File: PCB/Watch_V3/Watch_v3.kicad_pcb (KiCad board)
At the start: 2 copper layers, 39.1 x 63.2 mm, 102 parts, among them J1 USB_C_Receptacle_USB2.0_16P, J2 Screw_Terminal, J3 Peripheral, J4 OLED, J5 BN220, J6 Peripheral, J7 MAX30102, J8 ICSP, M1 Motor_DC, Q1 AO3401A, Q2 BC817, Q3 BC817, Q4 SI2302, Q5 BC847, SW1 SW_DPST_x2, SW2 SW_SPDT, SW3 SW_DPST_x2, SW4 Mode, SW5 Down, SW6 Select, SW7 Up, U1 AP2112K-3.3, U2 AP2112K-3.3, U3 TP4056, U4 ESP32-WROOM-32D, U5 CP2102N-Axx-xQFN28, U6 MPU-6050

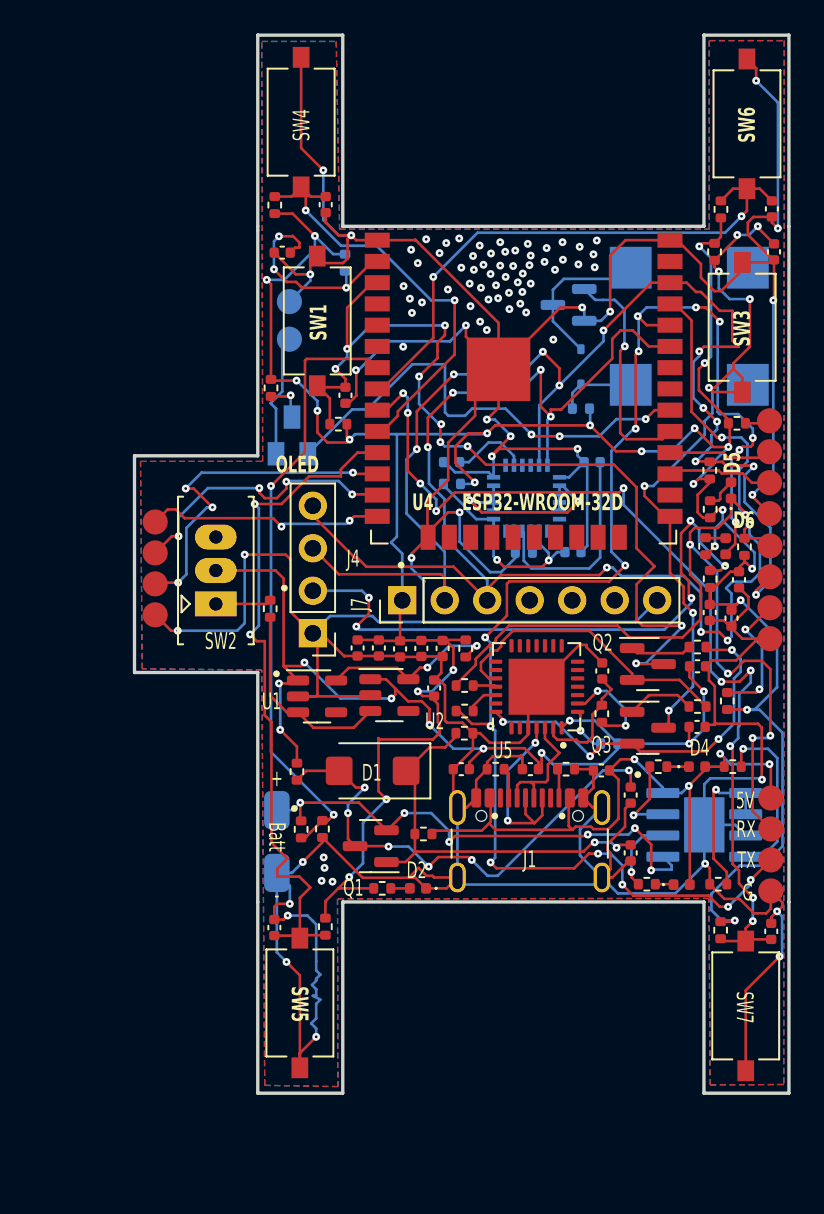
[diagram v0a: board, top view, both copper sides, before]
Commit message: update watch_v3
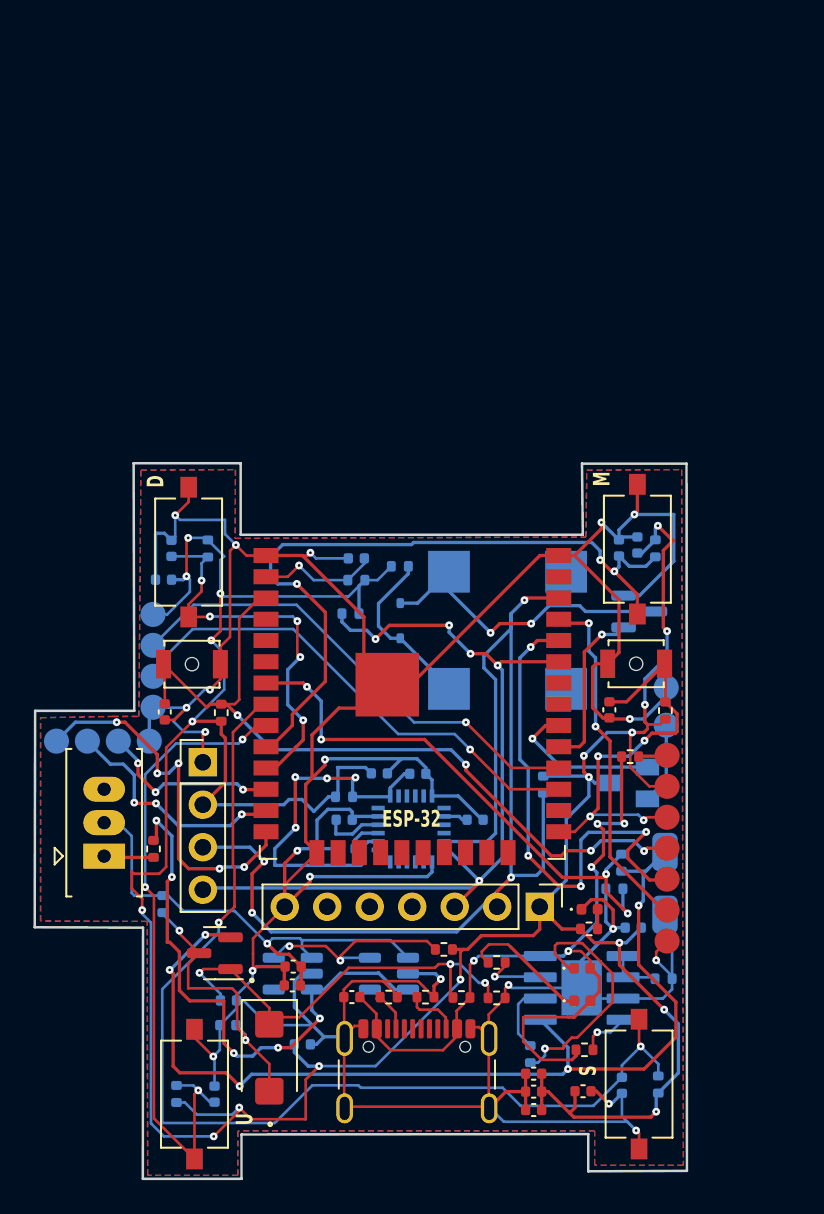
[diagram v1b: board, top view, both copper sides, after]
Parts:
- removed C4, C5, C6: 0.1uF, Capacitor_SMD:C_0402_1005Metric
- removed D5, D6: LED, LED_SMD:LED_0402_1005Metric
- removed G***: LOGO, Battery:xx
- removed G***: LOGO, Battery:robo2
- removed J6: Peripheral, Button_Switch_SMD:solder_pad_4
- removed Q2, Q3: BC817, Package_TO_SOT_SMD:SOT-23
- removed R10, R11: 150E, Resistor_SMD:R_0402_1005Metric
- removed R26, R27, R33, R37, R39: 0, Resistor_SMD:R_0402_1005Metric
- removed R30, R31: 220E, Resistor_SMD:R_0402_1005Metric
- removed R32: 4.7K, Resistor_SMD:R_0402_1005Metric
- removed R8: 1K, Resistor_SMD:R_0402_1005Metric
- removed U5: CP2102N-Axx-xQFN28, Package_DFN_QFN:QFN-28-1EP_5x5mm_P0.5mm_EP3.35x3.35mm
- C10, C11, C12, C17, C18, C2, C25, C26, C27, C28, C3, C9, J3, J5, R14, R15, R16, R17, R21, R22, R23, R24, R34, R5, R7, U1, U2: moved to B.Cu
- J8: value ICSP -> Conn_01x07_Pin; footprint Button_Switch_SMD:solder_pad_4 -> Button_Switch_SMD:solder_7
- R9: value 1K -> 0
- SW1, SW3: footprint Button_Switch_SMD:SW_Tactile_SPST_NO_Straight_CK_PTS636Sx25SMTRLFS -> Button_Switch_SMD:SW_SPST_B3U-1000P-B
- moved SW6 57.8 mm to (161.3, 103.8), turned to -90 degrees
- moved C27 53.2 mm to (160.3, 103.9)
- moved R23 52.4 mm to (162.5, 103.9)
- moved J5 44.0 mm to (129.5, 78.5)
- moved C28 34.7 mm to (136.0, 104.5)
- moved R24 34.0 mm to (133.7, 104.4), turned to -90 degrees
- moved SW7 33.4 mm to (134.8, 104.5), turned to 90 degrees
- moved SW4 32.5 mm to (161.2, 71.9)
- moved M1 32.2 mm to (160.5, 81.2)
- moved C20 31.7 mm to (155.1, 105.4), turned to 0 degrees
- moved R21 30.6 mm to (162.3, 71.8), turned to 90 degrees
- moved C19 30.5 mm to (155.1, 104.3), turned to 0 degrees
- moved C16 30.1 mm to (140.7, 96.8), turned to 180 degrees
- moved C8 29.1 mm to (159.6, 81.5)
- moved Q4 28.9 mm to (160.8, 85.8), turned to -90 degrees
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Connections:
- J1 pad A6: /D+ -> unconnected-(J1-D+-PadA6)
- J1 pad A7: /D- -> unconnected-(J1-D--PadA7)
- J1 pad B6: /D+ -> unconnected-(J1-D+-PadB6)
- J1 pad B7: /D- -> unconnected-(J1-D--PadB7)
- J4 pad 2: Net-(J4-Pin_2) -> +3.3V
- J5 pad 4: Net-(J5-Pin_4) -> +3.3V
- J8 pad 4: +5V -> /EN
- Q4 pad 3: Net-(Q4-Pad3) -> +3.3V
- R9 pad 1: Net-(Q3-B) -> +5V
- R9 pad 2: /RTS -> Net-(J8-Pin_7)
- U4 pad 34: /TX -> /RX
- U4 pad 35: /RX -> /TX
- U6 pad 15: unconnected-(U6-NC-Pad14) -> unconnected-(U6-NC-Pad15)
- U6 pad 16: unconnected-(U6-NC-Pad14) -> unconnected-(U6-NC-Pad16)
- U6 pad 17: unconnected-(U6-NC-Pad14) -> unconnected-(U6-NC-Pad17)
- U6 pad 2: unconnected-(U6-NC-Pad14) -> unconnected-(U6-NC-Pad2)
- U6 pad 3: unconnected-(U6-NC-Pad14) -> unconnected-(U6-NC-Pad3)
- U6 pad 4: unconnected-(U6-NC-Pad14) -> unconnected-(U6-NC-Pad4)
- U6 pad 5: unconnected-(U6-NC-Pad14) -> unconnected-(U6-NC-Pad5)
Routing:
- net GND: track 394.7 -> 268.3 mm, vias 87 -> 20
- net /TX: track 88.3 -> 21.0 mm, vias 16 -> 2
- net Net-(J4-Pin_2): track 36.3 -> 0.00 mm, vias 5 -> 0
- net /RX: track 66.4 -> 30.3 mm, vias 6 -> 4
- net VBUS: track 61.4 -> 29.7 mm, vias 10 -> 1
- net /Select: track 33.6 -> 63.6 mm
- net +BATT: track 30.4 -> 60.1 mm, vias 6 -> 5
- net /SDA: track 80.4 -> 50.9 mm, vias 8 -> 5
- net +3.3V: track 169.1 -> 193.6 mm, vias 24 -> 19
- net /TX2: track 6.22 -> 29.3 mm, vias 0 -> 1
- net /DTR: track 23.0 -> 0.00 mm, vias 4 -> 0
- net /RX2: track 6.33 -> 29.2 mm, vias 0 -> 1
- net ENA: track 11.9 -> 33.2 mm, vias 0 -> 5
- net /Up: track 58.5 -> 39.5 mm, vias 10 -> 3
- net /motor: track 28.3 -> 9.48 mm, vias 3 -> 1
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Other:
- board size 39.1 x 63.2 mm -> 39 x 42.8 mm
- board text added: "D"
- board text added: "ESP-32"
- board text added: "S"
- board text added: "U"
- board text removed: "+"
- board text removed: "-"
- board text removed: "3.3"
- board text removed: "5V"
- board text removed: "ARKA"
- board text removed: "Batt"
- board text removed: "C1"
- board text removed: "DHARMA ROBOFEST"
- board text removed: "ESP32-WROOM-32D"
- board text removed: "G"
- board text removed: "G12"
- board text removed: "G14"
- board text removed: "G27"
- board text removed: "KRS"
- board text removed: "RX"
- board text removed: "RX{dblquote}"
- board text removed: "SCL"
- board text removed: "SDA"
- board text removed: "SW1"
- board text removed: "SW3"
- board text removed: "TX"
- board text removed: "TX{dblquote}"
